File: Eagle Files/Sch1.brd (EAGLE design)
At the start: 62.2 x 53.3 mm, 14 parts

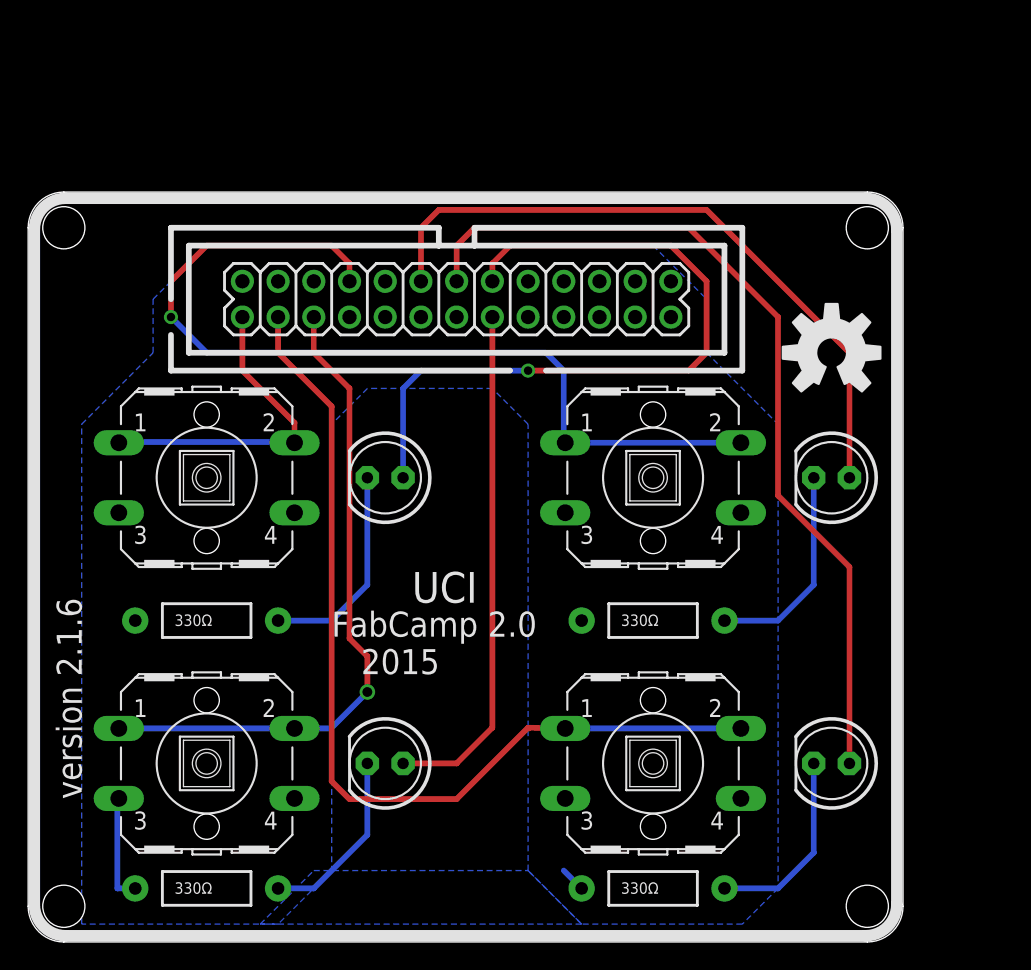
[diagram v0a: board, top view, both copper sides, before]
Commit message: Update Files
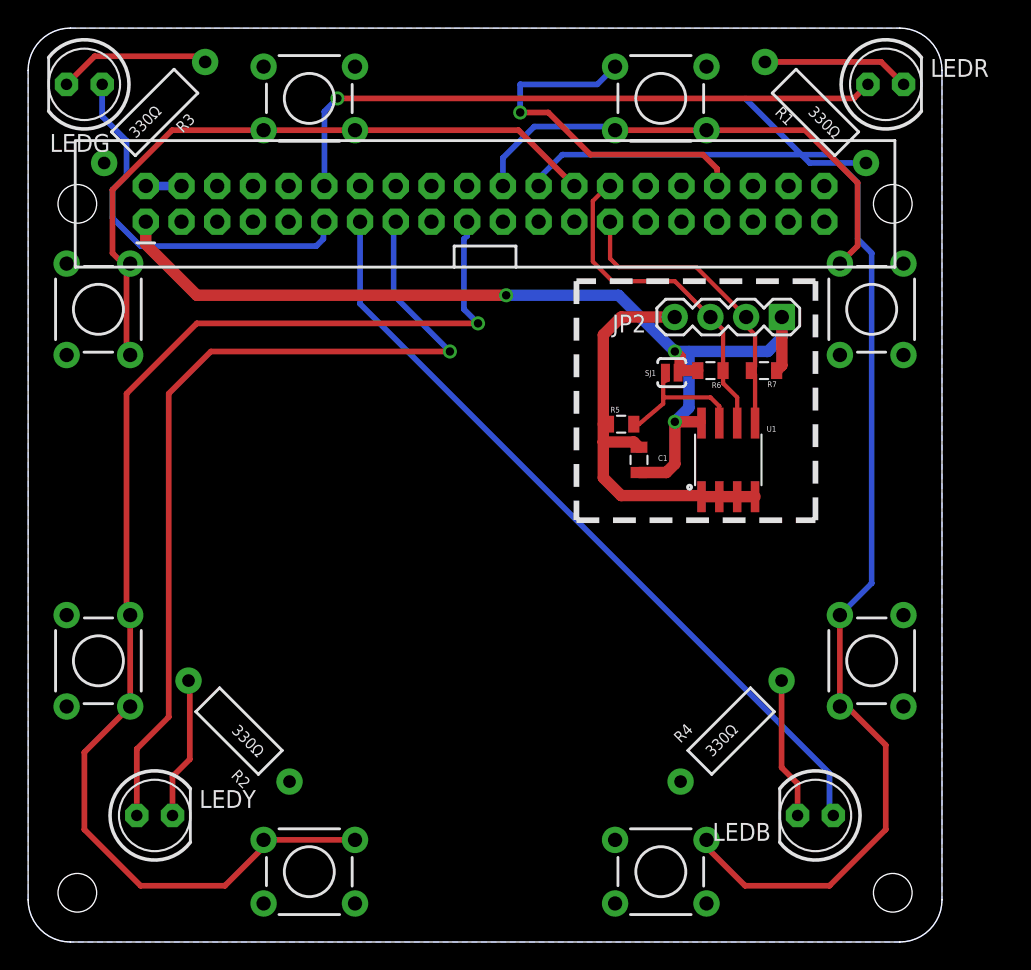
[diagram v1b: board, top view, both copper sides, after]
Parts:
- removed JP1K: M13X22X13, SparkFun-Connectors:2X13
- removed U$1: (no value), SparkFun-Aesthetics:OSHW-LOGO-L
- added C1, R5, R6, R7: (no value), SparkFun-Passives:0805
- added JP1: RASPBERRYPI-B+-GPIO, SparkFun-Boards:2X20-SHROUDED
- added JP2: (no value), SparkFun-Connectors:1X04
- added SB1, SG1, SR1, SY1: SWITCH-MOMENTARY-2PTH, SparkFun-Electromechanical:TACTILE-PTH
- added SJ1: SOLDERJUMPERNO, SparkFun-Retired:SJ_2S-NO
- added U1: EEPROM-I2CSMD, SparkFun-DigitalIC:SO08
- SB: value blue -> SWITCH-MOMENTARY-2PTH; device adafruit:B3F-40XX -> SparkFun-Electromechanical:TACTILE-PTH
- SG: value green -> SWITCH-MOMENTARY-2PTH; device adafruit:B3F-40XX -> SparkFun-Electromechanical:TACTILE-PTH
- SR: value red -> SWITCH-MOMENTARY-2PTH; device adafruit:B3F-40XX -> SparkFun-Electromechanical:TACTILE-PTH
- SY: value yellow -> SWITCH-MOMENTARY-2PTH; device adafruit:B3F-40XX -> SparkFun-Electromechanical:TACTILE-PTH
- moved R1 37.9 mm to (56.0, 59.0), turned to 135 degrees
- moved R3 36.3 mm to (9.00, 59.0), turned to 45 degrees
- moved LEDG 35.2 mm to (4.00, 61.0)
- moved LEDR 28.2 mm to (61.0, 61.0), turned to 0 degrees
- moved SG 28.0 mm to (20.0, 60.0)
- moved SR 19.6 mm to (60.0, 45.0), turned to 270 degrees
- moved LEDY 16.8 mm to (9.00, 9.00), turned to 0 degrees
- moved R4 12.5 mm to (50.0, 15.0), turned to 45 degrees
- moved R2 11.4 mm to (15.0, 15.0), turned to 135 degrees
- moved SY 10.6 mm to (20.0, 5.00), turned to 180 degrees
- moved SB 7.72 mm to (45.0, 5.00), turned to 180 degrees
- moved LEDB 3.87 mm to (56.0, 9.00)
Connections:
- new net 3.3V: JP1.17
- new net 5V: JP1.2, JP1.4
- new net N$5: JP1.27, JP2.2, R7.1, U1.5
- new net N$6: JP1.28, JP2.3, R6.1, U1.6
- new net N$8: R5.2, SJ1.1, U1.7
- new net VCC: C1.1, JP1.1, JP2.1, R6.2, R7.2, SJ1.2, U1.8
- net GND: now also C1.2, JP1.14, JP1.20, JP1.25, JP1.30, JP1.33, JP1.34, JP1.39, JP1.6, JP1.9, JP2.4, R5.1, SB.1, SB1.1, SG.1, SG1.1, SR.1, SR1.1, SY.1, SY1.1, U1.1, U1.2, U1.3, U1.4; no longer JP1K.6, SB.3, SB.4, SG.3, SG.4, SR.3, SR.4, SY.3, SY.4
- net LB: now also JP1.13; no longer JP1K.13
- net LG: now also JP1.11; no longer JP1K.11
- net LR: now also JP1.12; no longer JP1K.15
- net LY: now also JP1.15; no longer JP1K.12
- net SB: now also JP1.24, SB.3, SB1.3; no longer JP1K.24, SB.1, SB.2
- net SG: now also JP1.26, SG.3, SG1.3; no longer JP1K.26, SG.1, SG.2
- net SR: now also JP1.22, SR.3, SR1.3; no longer JP1K.19, SR.1, SR.2
- net SY: now also JP1.19, SY.3, SY1.3; no longer JP1K.22, SY.1, SY.2
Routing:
- net VCC: track 0.00 -> 72.0 mm, vias 0 -> 3
- net GND: track 9.80 -> 66.8 mm, vias 0 -> 1
- net SY: track 47.2 -> 89.5 mm
- net SR: track 65.4 -> 36.1 mm, vias 1 -> 0
- net LY: track 36.6 -> 63.1 mm, vias 0 -> 1
- net SG: track 23.2 -> 48.5 mm
- net N$6: track 0.00 -> 24.3 mm
- net LG: track 52.2 -> 27.9 mm, vias 1 -> 0
- net SB: track 66.4 -> 89.7 mm
- net N$5: track 0.00 -> 22.0 mm
- net N$8: track 0.00 -> 10.5 mm
- net LB: track 62.4 -> 56.2 mm
- net N$1: track 15.0 -> 10.5 mm
- net N$3: track 15.0 -> 10.9 mm
- net N$4: track 13.8 -> 10.1 mm
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- removed copper zone on layer 16, net N$5
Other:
- board size 62.2 x 53.3 mm -> 65 x 65 mm
- board text removed: "FabCamp 2.0 2015"
- board text removed: "UCI"
- board text removed: "version 2.1.6"
